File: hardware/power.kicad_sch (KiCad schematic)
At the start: 3 parts, among them J1 USB_C_Receptacle_USB2.0_16P, U3 MCP73871-2CC, U4 MCP1700x-330xxTT

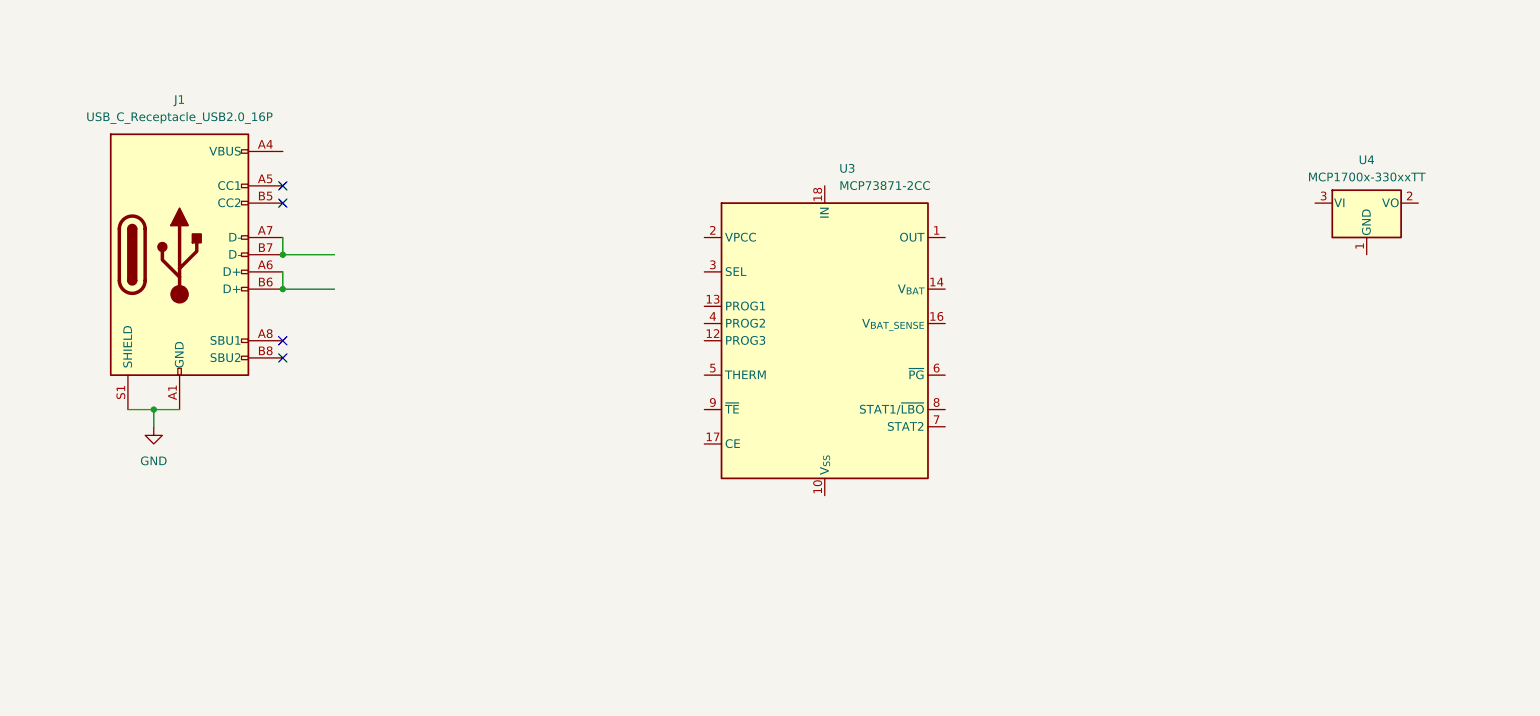
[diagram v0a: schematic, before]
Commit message: wip: power circuit
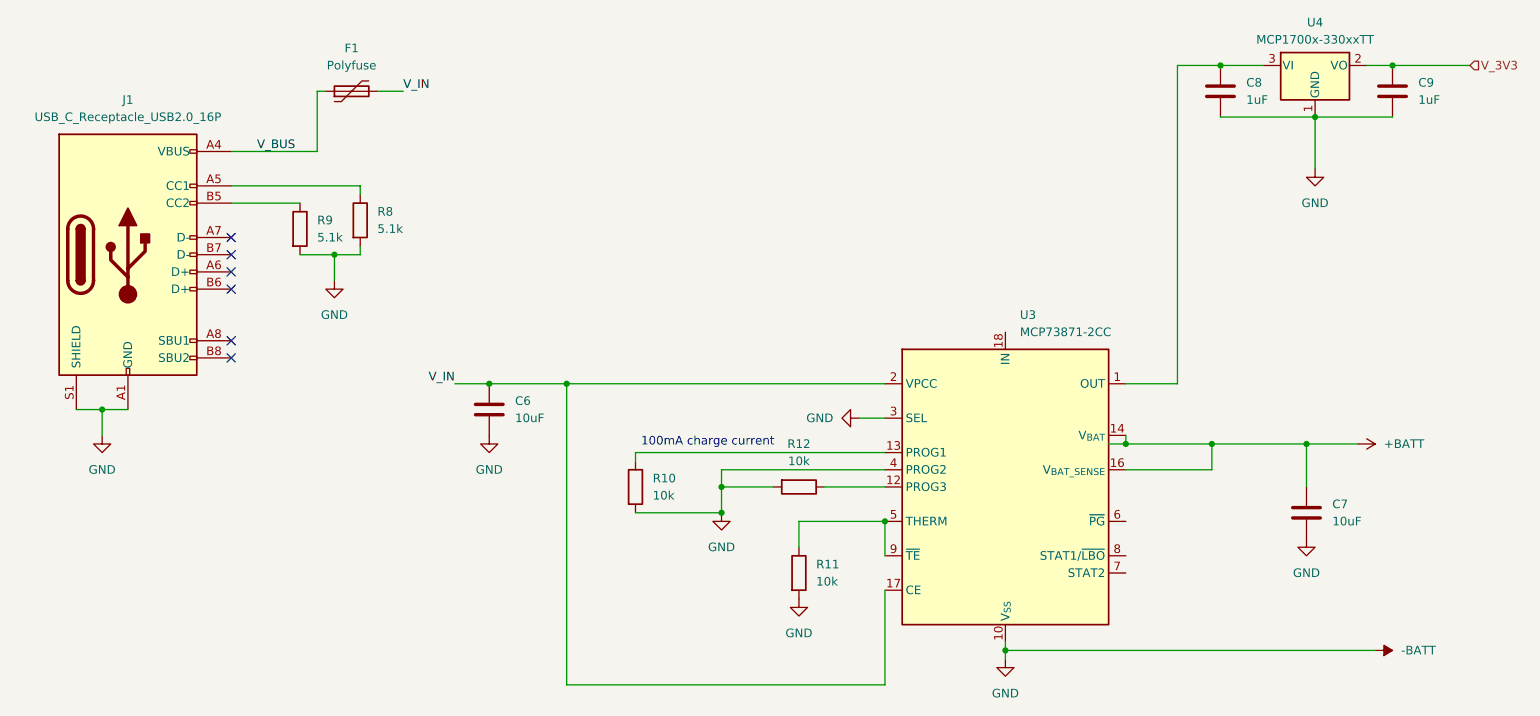
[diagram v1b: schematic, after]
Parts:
- added C6, C7: 10uF, symbol Device:C
- added C8, C9: 1uF, symbol Device:C
- added F1: Polyfuse, symbol Device:Polyfuse
- added R10, R11, R12: 10k, symbol Device:R
- added R8, R9: 5.1k, symbol Device:R
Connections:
- net GND is gone; now on net -BATT: J1.A1 (GND), J1.A12 (GND), J1.B1 (GND), J1.B12 (GND), J1.S1 (SHIELD)
- net -BATT: now reaches U4.1 (GND)
- net -BATT: now also U3.10 (V_{SS}), U3.11 (V_{SS}), U3.21 (V_{SS}), U3.3 (SEL), U3.4 (PROG2), C6.2, C7.2, C8.2, C9.2, R10.2, R11.2, R12.2, R8.2, R9.2
- net V_3V3: now reaches U4.2 (VO)
- net V_3V3: now also C9.1
- net at U4.3 (VI): now also U3.1 (OUT), U3.20 (OUT), C8.1
- net V_BUS: now reaches J1.A4 (VBUS), J1.A9 (VBUS), J1.B4 (VBUS), J1.B9 (VBUS)
- net V_BUS: now also F1.1
- net at J1.A5 (CC1): now also R8.1
- net at J1.A6 (D+): no longer J1.B6 (D+)
- net at J1.A7 (D-): no longer J1.B7 (D-)
- net at J1.B5 (CC2): now also R9.1
- net at U3.12 (PROG3): now also R12.1
- net at U3.13 (PROG1): now also R10.1
- net +BATT: now reaches U3.14 (V_{BAT}), U3.15 (V_{BAT})
- net +BATT: now also U3.16 (V_{BAT_SENSE}), C7.1
- net V_IN: now reaches U3.17 (CE)
- net V_IN: now also U3.2 (VPCC), C6.1, F1.2
- net at U3.5 (THERM): now also U3.9 (~{TE}), R11.1
- no-connect marks 4 -> 6
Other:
- note added: "100mA charge current"
- moved on the sheet: J1, U3, U4
